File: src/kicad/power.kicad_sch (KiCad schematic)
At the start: 36 parts, among them J2 USB_C_Receptacle_USB2.0_16P, J5 Conn_01x02, Q2 BSS138, Q3 BSS138, SW1 EVQPUL02K, U7 TPS63070RNMR, U8 BQ24075RGT, U9 MAX17048G_T10

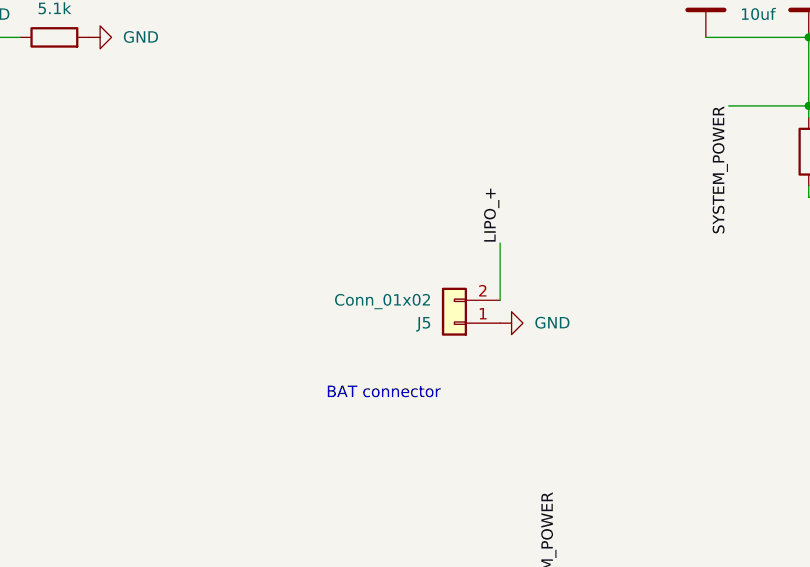
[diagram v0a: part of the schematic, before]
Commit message: may 29th + files updates
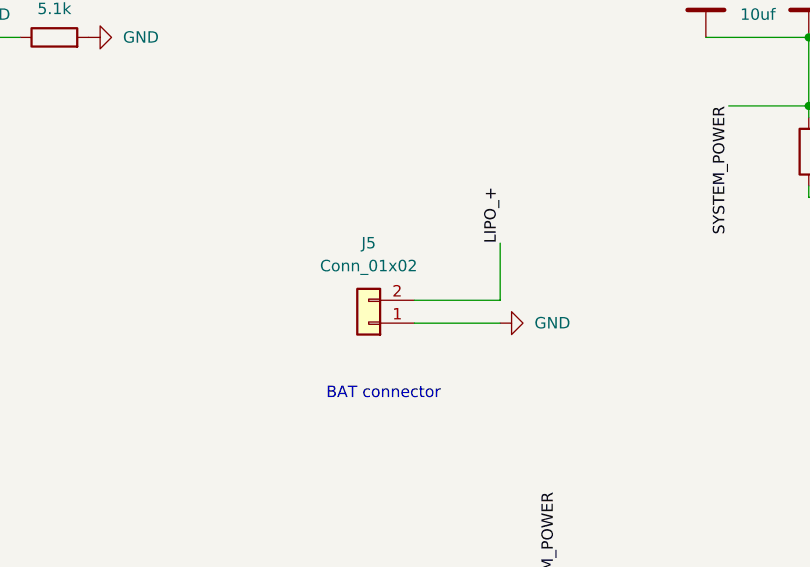
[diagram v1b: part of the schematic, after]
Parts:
- C27: footprint (none) -> Capacitor_SMD:C_0402_1005Metric; LCSC Part (none) -> C1525
- C28, C30: footprint (none) -> Capacitor_SMD:C_0603_1608Metric; LCSC Part (none) -> C19666
- C29: footprint (none) -> Capacitor_SMD:C_0402_1005Metric; LCSC Part (none) -> C52923
- C31, C33, C37, C38: footprint (none) -> Capacitor_SMD:C_0603_1608Metric; LCSC Part (none) -> C96446
- C34, C35, C36: footprint (none) -> Capacitor_SMD:C_0603_1608Metric; LCSC Part (none) -> C59461
- D2, D3: footprint (none) -> Diode_SMD:D_SOD-123; LCSC Part (none) -> C8598
- J5: footprint (none) -> Connector_JST:JST_PH_S2B-PH-SM4-TB_1x02-1MP_P2.00mm_Horizontal; LCSC Part (none) -> C295747
- L2: footprint (none) -> Inductor_SMD:L_Sunlord_MWSA0402S; LCSC Part (none) -> C408334
